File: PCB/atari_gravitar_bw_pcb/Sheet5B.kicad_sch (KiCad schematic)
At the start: 0 parts

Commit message: Finished sheet 5B
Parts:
- added J_3: 74LS04, symbol atari:74LS04
- added J_6, M_5: 74LS32, symbol atari:74LS32
- added J_7: 74LS139, symbol atari:74LS139
- added K_7: 6116, symbol atari:6116
- added K_8, L_8, M_8, N_8: 74LS157, symbol atari:74LS157
- added L_7, M/N_7, N/P_7, R_7: 2732, symbol atari:2732
- added P_8: 74LS245, symbol atari:74LS245
- added R61, R62, R63, R64, R65, R66, R67, R68: 10k, symbol Device:R_US
- added TPSAEN1, TPVRAM1, TPVROM0, TPVROM1, TPVROM2, TPVROM3: tp_2_pin, symbol atari:tp_2_pin
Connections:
- new net: J_6.13, K_8.9 (Zc)
- new net: M_5.8, TPSAEN1.1, TPSAEN1.2
- new net: J_3.4, M_5.9
- new net: J_7.13 (A1), M_8.4 (Za)
- new net: J_7.1 (E), J_7.12 (O3)
- new net: J_7.14 (A0), K_8.4 (Za)
- new net +5V: J_7.16 (VCC), K_7.24 (VCC), K_8.16 (VCC), L_7.21 (VPP), L_7.24 (VCC), L_8.16 (VCC), M/N_7.21 (VPP), M/N_7.24 (VCC), M_8.16 (VCC), N/P_7.21 (VPP), N/P_7.24 (VCC), N_8.16 (VCC), P_8.20 (VCC), R61.1, R62.1, R63.1, R64.1, R65.1, R66.1, R67.1, R68.1, R_7.21 (VPP), R_7.24 (VCC)
- new net AB0: N_8.14 (I0d)
- new net AB1: N_8.11 (I0c)
- new net AB10: M_8.14 (I0d)
- new net AB11: K_8.14 (I0d)
- new net AB12: K_8.2 (I0a)
- new net AB2: N_8.2 (I0a)
- new net AB3: N_8.5 (I0b)
- new net AB4: L_8.2 (I0a)
- new net AB5: L_8.5 (I0b)
- new net AB6: L_8.11 (I0c)
- new net AB7: L_8.14 (I0d)
- new net AB8: M_8.5 (I0b)
- new net AB9: M_8.11 (I0c)
- new net AM0: K_7.8 (A0), N_8.12 (Zd), R_7.8 (A0)
- new net AM1: K_7.7 (A1), N_8.9 (Zc), R_7.7 (A1)
- new net AM10: J_3.3, K_7.19 (A10), M_8.12 (Zd), R_7.19 (A10)
- new net AM11: J_7.2 (A0), K_8.12 (Zd), R_7.18 (A11)
- new net AM2: K_7.6 (A2), N_8.4 (Za), R_7.6 (A2)
- new net AM3: K_7.5 (A3), N_8.7 (Zb), R_7.5 (A3)
- new net AM4: K_7.4 (A4), L_8.4 (Za), R_7.4 (A4)
- new net AM5: K_7.3 (A5), L_8.7 (Zb), R_7.3 (A5)
- new net AM6: K_7.2 (A6), L_8.9 (Zc), R_7.2 (A6)
- new net AM7: K_7.1 (A7), L_8.12 (Zd), R_7.1 (A7)
- new net AM8: K_7.23 (A8), M_8.7 (Zb), R_7.23 (A8)
- new net AM9: K_7.22 (A9), M_8.9 (Zc), R_7.22 (A9)
- new net AVG0: N_8.13 (I1d)
- new net AVG1: N_8.10 (I1c)
- new net AVG10: M_8.13 (I1d)
- new net AVG11: K_8.13 (I1d)
- new net AVG12: K_8.3 (I1a)
- new net AVG13: M_8.3 (I1a)
- new net AVG2: N_8.3 (I1a)
- new net AVG3: N_8.6 (I1b)
- new net AVG4: L_8.3 (I1a)
- new net AVG5: L_8.6 (I1b)
- new net AVG6: L_8.10 (I1c)
- new net AVG7: L_8.13 (I1d)
- new net AVG8: M_8.6 (I1b)
- new net AVG9: M_8.10 (I1c)
- new net DB0: P_8.3
- new net DB1: P_8.2
- new net DB2: P_8.4
- new net DB3: P_8.5
- new net DB4: P_8.6
- new net DB5: P_8.9
- new net DB6: P_8.8
- new net DB7: P_8.7
- new net DVG0: K_7.9 (D0), L_7.9 (D0), P_8.17, R66.2
- new net DVG1: K_7.10 (D1), L_7.10 (D1), P_8.18, R67.2
- new net DVG2: K_7.11 (D2), L_7.11 (D2), P_8.16, R68.2
- new net DVG3: K_7.13 (D3), L_7.13 (D3), P_8.15, R65.2
- new net DVG4: K_7.14 (D4), L_7.14 (D4), P_8.14, R64.2
- new net DVG5: K_7.15 (D5), L_7.15 (D5), P_8.11, R63.2
- new net DVG6: K_7.16 (D6), L_7.16 (D6), P_8.12, R62.2
- new net DVG7: K_7.17 (D7), L_7.17 (D7), P_8.13, R61.2
- new net GND: J_7.15 (E), J_7.3 (A1), J_7.8 (GND), K_7.12 (GND), K_7.20 (~{OE}), K_8.15 (E), K_8.8 (GND), L_7.12 (GND), L_8.15 (E), L_8.8 (GND), M/N_7.12 (GND), M_8.15 (E), M_8.8 (GND), N/P_7.12 (GND), N_8.15 (E), N_8.8 (GND), P_8.10 (GND), R_7.12 (GND)
- new net PR82: K_8.10 (I1c), K_8.6 (I1b)
- new net ~{AB13}: M_8.2 (I0a)
- new net ~{BPHI2}: J_6.12, K_8.5 (I0b)
- new net ~{BUFFEN}: K_8.7 (Zb), P_8.19 (G)
- new net ~{R}WB: P_8.1 (D/R)
- new net ~{VMEM}: K_8.1 (S), L_8.1 (S), M_8.1 (S), N_8.1 (S)
- new net ~{VRAM}: J_7.4 (O0), K_7.18 (~{CE}), M_5.10, TPVRAM1.1, TPVRAM1.2
- new net ~{VROM0}: J_7.5 (O1), L_7.20 (~{CS}), TPVROM0.1, TPVROM0.2
- new net ~{VROM1}: J_7.11 (O2), M/N_7.20 (~{CS}), TPVROM1.1, TPVROM1.2
- new net ~{VROM2}: J_7.10 (O1), N/P_7.20 (~{CS}), TPVROM2.1, TPVROM2.2
- new net ~{VROM3}: J_7.9 (O0), R_7.20 (~{CS}), TPVROM3.1, TPVROM3.2
- new net ~{VW}: J_6.11, K_7.21 (~{WE})
- new net ~{WRITE}: K_8.11 (I0c)
- no-connect marks 0 -> 2
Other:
- note added: "VECTOR ADDRESS DECODER"
- note added: "VECTOR ADDRESS SELECTOR"
- note added: "VECTOR MEMORY DATA BUFFER"
- note added: "VECTOR RANDOM-ACCESS MEMORY"
- note added: "VECTOR READ-ONLY MEMORY"

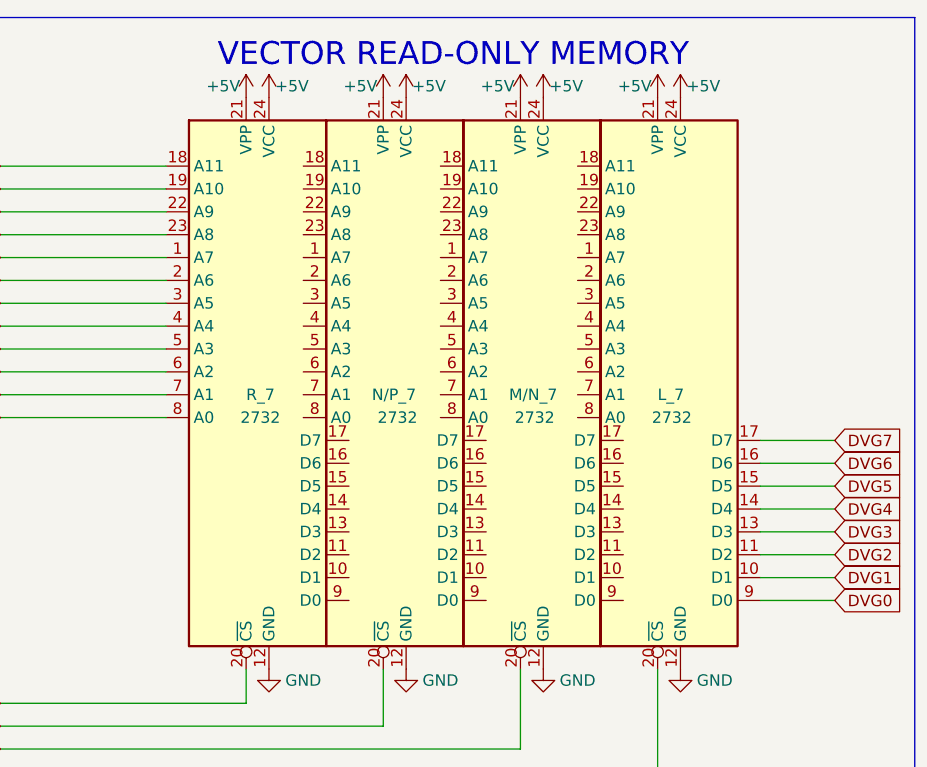
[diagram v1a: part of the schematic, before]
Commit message: Finished sheet 6A
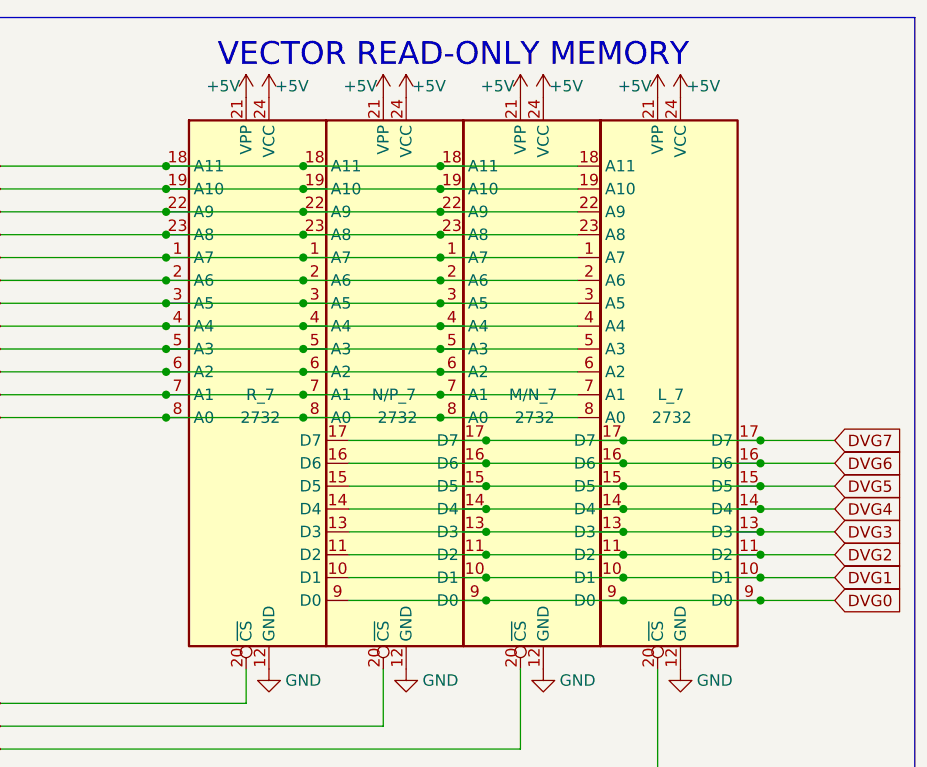
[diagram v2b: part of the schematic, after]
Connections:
- net AM0: now also L_7.8 (A0), M/N_7.8 (A0), N/P_7.8 (A0)
- net AM1: now also L_7.7 (A1), M/N_7.7 (A1), N/P_7.7 (A1)
- net AM10: now also L_7.19 (A10), M/N_7.19 (A10), N/P_7.19 (A10)
- net AM11: now also L_7.18 (A11), M/N_7.18 (A11), N/P_7.18 (A11)
- net AM2: now also L_7.6 (A2), M/N_7.6 (A2), N/P_7.6 (A2)
- net AM3: now also L_7.5 (A3), M/N_7.5 (A3), N/P_7.5 (A3)
- net AM4: now also L_7.4 (A4), M/N_7.4 (A4), N/P_7.4 (A4)
- net AM5: now also L_7.3 (A5), M/N_7.3 (A5), N/P_7.3 (A5)
- net AM6: now also L_7.2 (A6), M/N_7.2 (A6), N/P_7.2 (A6)
- net AM7: now also L_7.1 (A7), M/N_7.1 (A7), N/P_7.1 (A7)
- net AM8: now also L_7.23 (A8), M/N_7.23 (A8), N/P_7.23 (A8)
- net AM9: now also L_7.22 (A9), M/N_7.22 (A9), N/P_7.22 (A9)
- net DVG0: now also M/N_7.9 (D0), N/P_7.9 (D0), R_7.9 (D0)
- net DVG1: now also M/N_7.10 (D1), N/P_7.10 (D1), R_7.10 (D1)
- net DVG2: now also M/N_7.11 (D2), N/P_7.11 (D2), R_7.11 (D2)
- net DVG3: now also M/N_7.13 (D3), N/P_7.13 (D3), R_7.13 (D3)
- net DVG4: now also M/N_7.14 (D4), N/P_7.14 (D4), R_7.14 (D4)
- net DVG5: now also M/N_7.15 (D5), N/P_7.15 (D5), R_7.15 (D5)
- net DVG6: now also M/N_7.16 (D6), N/P_7.16 (D6), R_7.16 (D6)
- net DVG7: now also M/N_7.17 (D7), N/P_7.17 (D7), R_7.17 (D7)
